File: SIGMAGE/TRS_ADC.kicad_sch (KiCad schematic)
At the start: 32 parts, among them J2 SJ63073E, J3 SJ63073E, J4 SJ63073E, J5 SJ63073E, U4 OPA1612AIDRGR, U5 PCM1803ADB, U6 OPA1612AIDRGR, U7 PCM1803ADB

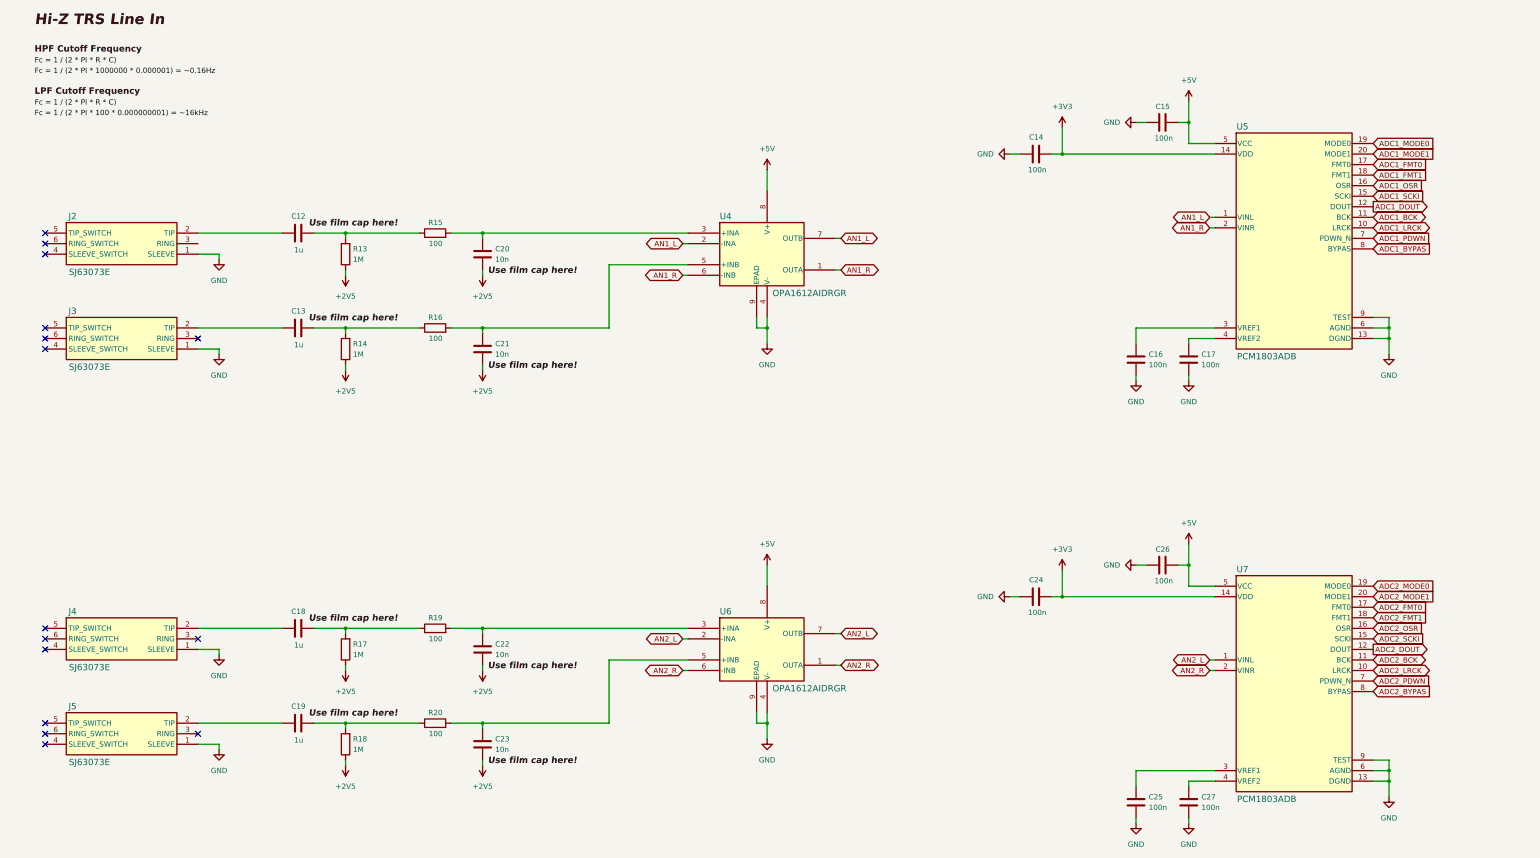
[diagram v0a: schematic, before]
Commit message: Finished schematic
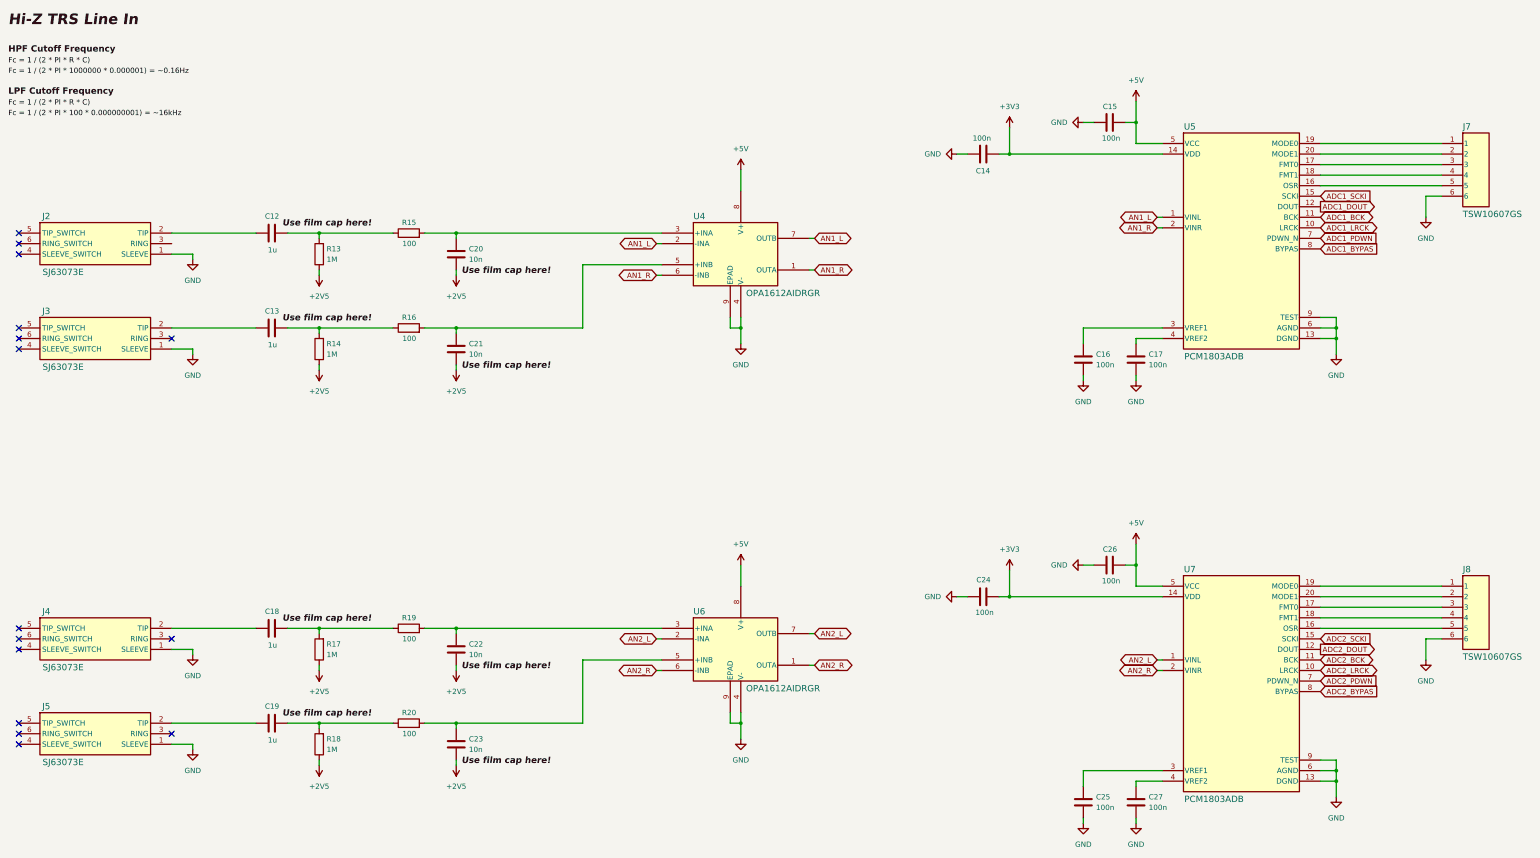
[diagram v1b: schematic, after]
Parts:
- added J7, J8: TSW10607GS, SIGMAGE:TSW10607GS, symbol SIGMAGE:TSW10607GS
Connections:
- net +3V3: now also C14.1; no longer C14.2
- net GND: now also C14.2, J7.6, J8.6; no longer C14.1
- net ADC1_FMT0: no longer names the net of U5.17 (FMT0)
- net ADC1_FMT0: now also J7.3
- net ADC1_FMT1: no longer names the net of U5.18 (FMT1)
- net ADC1_FMT1: now also J7.4
- net ADC1_MODE0: no longer names the net of U5.19 (MODE0)
- net ADC1_MODE0: now also J7.1
- net ADC1_MODE1: no longer names the net of U5.20 (MODE1)
- net ADC1_MODE1: now also J7.2
- net ADC1_OSR: no longer names the net of U5.16 (OSR)
- net ADC1_OSR: now also J7.5
- net ADC2_FMT0: no longer names the net of U7.17 (FMT0)
- net ADC2_FMT0: now also J8.3
- net ADC2_FMT1: no longer names the net of U7.18 (FMT1)
- net ADC2_FMT1: now also J8.4
- net ADC2_MODE0: no longer names the net of U7.19 (MODE0)
- net ADC2_MODE0: now also J8.1
- net ADC2_MODE1: no longer names the net of U7.20 (MODE1)
- net ADC2_MODE1: now also J8.2
- net ADC2_OSR: no longer names the net of U7.16 (OSR)
- net ADC2_OSR: now also J8.5
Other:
- moved on the sheet: C12, C13, C14, C15, C16, C17, C18, C19, C20, C21, C22, C23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
